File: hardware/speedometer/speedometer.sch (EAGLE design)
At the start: 128 parts, among them IC1 PIC32MX274F256DT-I_PT, IC10 TPS63001DRCT, IC11 TPS63002DRCT, IC2 CSTCE8M00G55-R0, IC3 HM-11, IC4 BQ27441DRZR-G1A, IC5 BQ24075RGTT, IC6 NRF24L01P-T, IC7 CSTCE16M0V53-R0, IC8 24LC024SN, IC9 MAX16054AZT+T, J1 10104111-0001LF, J2 BAT, J3 CONUFL001-SMD-T, J4 Right_sens, J5 Right, J6 Left_sens, J7 Left, Q1 BC817, Q2 BC817, Q3 BC817, Q4 BC817, U1 SN74AHC1G08DBVR, U2 SN74AHC1G08DBVR, X1 TSW-102-07-G-S, X2 TSW-102-07-G-S

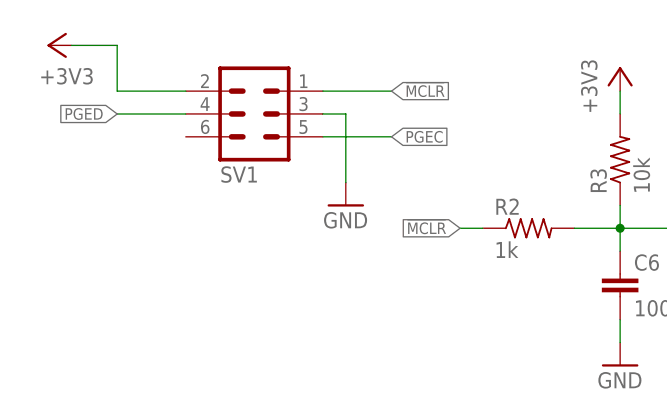
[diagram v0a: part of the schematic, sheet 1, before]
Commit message: wip
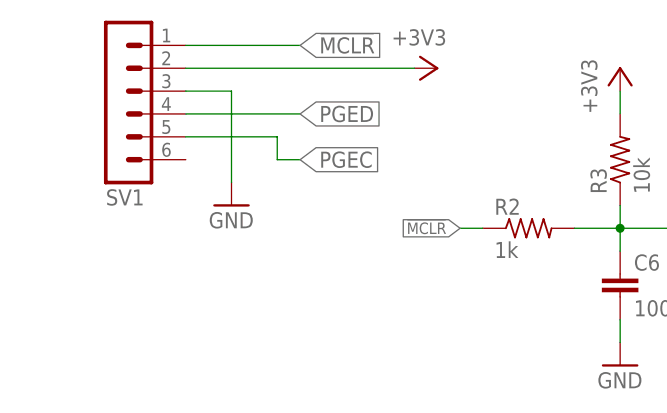
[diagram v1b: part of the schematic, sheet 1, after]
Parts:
- C3: device rcl:C-EUC0603K -> rcl:C-EUC0805K
- SV1: device con-lstb:MA03-2 -> con-lstb:MA06-1
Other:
- moved on the sheet: SV1
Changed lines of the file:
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@@
 <part name="GND11" library="supply1" library_urn="urn:adsk.eagle:library:371" deviceset="GND" device=""/>
 <part name="VDD1" library="supply1" library_urn="urn:adsk.eagle:library:371" deviceset="VDD" device=""/>
-<part name="C3" library="rcl" library_urn="urn:adsk.eagle:library:334" deviceset="C-EU" device="C0603K" value="10u"/>
+<part name="C3" library="rcl" library_urn="urn:adsk.eagle:library:334" deviceset="C-EU" device="C0805K" package3d_urn="urn:adsk.eagle:package:23681/2" value="10u"/>
 <part name="GND2" library="supply1" library_urn="urn:adsk.eagle:library:371" deviceset="GND" device=""/>
 <part name="C1" library="rcl" library_urn="urn:adsk.eagle:library:334" deviceset="C-EU" device="C0603K" value="100n"/>
@@
 <part name="GND63" library="supply1" library_urn="urn:adsk.eagle:library:371" deviceset="GND" device=""/>
 <part name="+3V2" library="supply1" library_urn="urn:adsk.eagle:library:371" deviceset="+3V3" device=""/>
-<part name="SV1" library="con-lstb" library_urn="urn:adsk.eagle:library:162" deviceset="MA03-2" device="" package3d_urn="urn:adsk.eagle:package:8334/1"/>
 <part name="X1" library="con-samtec" library_urn="urn:adsk.eagle:library:184" deviceset="TSW-102-*-G-S" device="" technology="07"/>
 <part name="X2" library="con-samtec" library_urn="urn:adsk.eagle:library:184" deviceset="TSW-102-*-G-S" device="" technology="07"/>
 <part name="GND64" library="supply1" library_urn="urn:adsk.eagle:library:371" deviceset="GND" device=""/>
+<part name="SV1" library="con-lstb" library_urn="urn:adsk.eagle:library:162" deviceset="MA06-1" device="" package3d_urn="urn:adsk.eagle:package:8340/1"/>
 </parts>
 <sheets>
@@
 <attribute name="SHEET" x="230.505" y="5.08" size="2.54" layer="94"/>
 </instance>
-<instance part="GND1" gate="1" x="40.64" y="149.86" smashed="yes">
-<attribute name="VALUE" x="38.1" y="147.32" size="1.778" layer="96"/>
-</instance>
-<instance part="+3V34" gate="G$1" x="7.62" y="167.64" smashed="yes" rot="R90">
-<attribute name="VALUE" x="12.7" y="165.1" size="1.778" layer="96" rot="R180"/>
+<instance part="GND1" gate="1" x="27.94" y="149.86" smashed="yes">
+<attribute name="VALUE" x="25.4" y="147.32" size="1.778" layer="96"/>
+</instance>
+<instance part="+3V34" gate="G$1" x="50.8" y="165.1" smashed="yes" rot="R270">
+<attribute name="VALUE" x="45.72" y="167.64" size="1.778" layer="96"/>
 </instance>
 <instance part="TP8" gate="G$1" x="236.22" y="139.7" smashed="yes">
@@
 <attribute name="VALUE" x="34.29" y="50.038" size="1.778" layer="96"/>
 </instance>
-<instance part="SV1" gate="1" x="30.48" y="160.02" smashed="yes" rot="MR180">
-<attribute name="VALUE" x="26.67" y="167.64" size="1.778" layer="96" rot="MR180"/>
-<attribute name="NAME" x="26.67" y="154.178" size="1.778" layer="95" rot="MR180"/>
-</instance>
 <instance part="X1" gate="-1" x="95.25" y="142.24" smashed="yes">
 <attribute name="VALUE" x="93.98" y="143.51" size="1.778" layer="96"/>
@@
 <instance part="X2" gate="-2" x="110.49" y="27.94" smashed="yes">
 <attribute name="NAME" x="113.03" y="27.178" size="1.524" layer="95"/>
+</instance>
+<instance part="SV1" gate="1" x="15.24" y="160.02" smashed="yes" rot="MR180">
+<attribute name="VALUE" x="13.97" y="172.72" size="1.778" layer="96" rot="MR180"/>
+<attribute name="NAME" x="13.97" y="151.638" size="1.778" layer="95" rot="MR180"/>
 </instance>
 </instances>
@@
 <segment>
 <pinref part="SV1" gate="1" pin="3"/>
-<wire x1="38.1" y1="160.02" x2="40.64" y2="160.02" width="0.1524" layer="91"/>
+<wire x1="22.86" y1="162.56" x2="27.94" y2="162.56" width="0.1524" layer="91"/>
 <pinref part="GND1" gate="1" pin="GND"/>
-<wire x1="40.64" y1="160.02" x2="40.64" y2="152.4" width="0.1524" layer="91"/>
+<wire x1="27.94" y1="162.56" x2="27.94" y2="152.4" width="0.1524" layer="91"/>
 </segment>
 </net>
@@
 </segment>
 <segment>
+<pinref part="SV1" gate="1" pin="2"/>
 <pinref part="+3V34" gate="G$1" pin="+3V3"/>
-<wire x1="10.16" y1="167.64" x2="15.24" y2="167.64" width="0.1524" layer="91"/>
-<wire x1="15.24" y1="167.64" x2="15.24" y2="162.56" width="0.1524" layer="91"/>
-<pinref part="SV1" gate="1" pin="2"/>
-<wire x1="15.24" y1="162.56" x2="22.86" y2="162.56" width="0.1524" layer="91"/>
+<wire x1="22.86" y1="165.1" x2="48.26" y2="165.1" width="0.1524" layer="91"/>
 </segment>
 </net>
@@
 <segment>
 <pinref part="SV1" gate="1" pin="5"/>
-<wire x1="38.1" y1="157.48" x2="45.72" y2="157.48" width="0.1524" layer="91"/>
-<label x="45.72" y="157.48" size="1.27" layer="95" font="vector" xref="yes"/>
+<wire x1="22.86" y1="157.48" x2="33.02" y2="157.48" width="0.1524" layer="91"/>
+<wire x1="33.02" y1="157.48" x2="33.02" y2="154.94" width="0.1524" layer="91"/>
+<wire x1="33.02" y1="154.94" x2="35.56" y2="154.94" width="0.1524" layer="91"/>
+<label x="35.56" y="154.94" size="1.778" layer="95" font="vector" xref="yes"/>
 </segment>
 </net>
@@
 <segment>
 <pinref part="SV1" gate="1" pin="4"/>
-<wire x1="22.86" y1="160.02" x2="15.24" y2="160.02" width="0.1524" layer="91"/>
-<label x="15.24" y="160.02" size="1.27" layer="95" font="vector" rot="R180" xref="yes"/>
+<wire x1="22.86" y1="160.02" x2="35.56" y2="160.02" width="0.1524" layer="91"/>
+<label x="35.56" y="160.02" size="1.778" layer="95" font="vector" xref="yes"/>
 </segment>
 </net>
@@
 <segment>
 <pinref part="SV1" gate="1" pin="1"/>
-<wire x1="38.1" y1="162.56" x2="45.72" y2="162.56" width="0.1524" layer="91"/>
-<label x="45.72" y="162.56" size="1.27" layer="95" font="vector" xref="yes"/>
-</segment>
-</net>
+<wire x1="22.86" y1="167.64" x2="35.56" y2="167.64" width="0.1524" layer="91"/>
+<label x="35.56" y="167.64" size="1.778" layer="95" font="vector" xref="yes"/>
+</segment>
+</net>
